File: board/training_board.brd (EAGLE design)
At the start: 68.6 x 53.4 mm, 24 parts, among them J1 MAIN_PWR, Q1 ARDUINOR3-NOIOREF-NOTEXT, Q2 DMN2056U, SW2 PTS645, U1 DRV8871HSOP-8

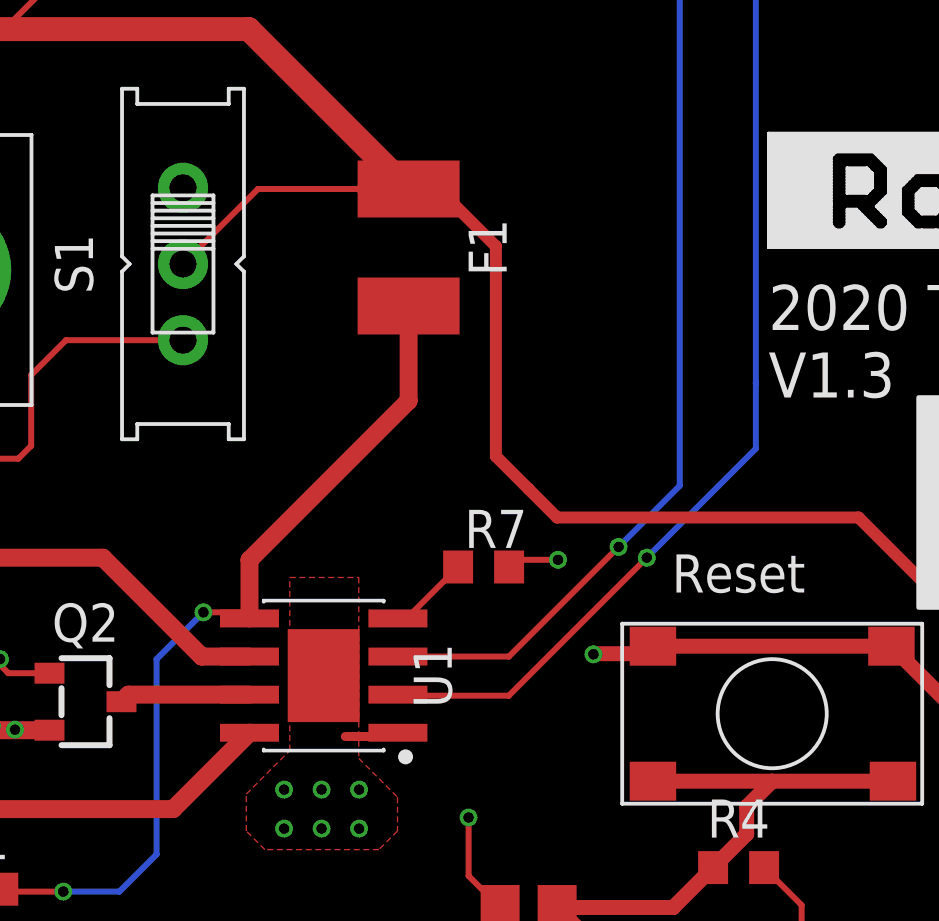
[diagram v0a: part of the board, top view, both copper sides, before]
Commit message: Library updates, slight routing changes
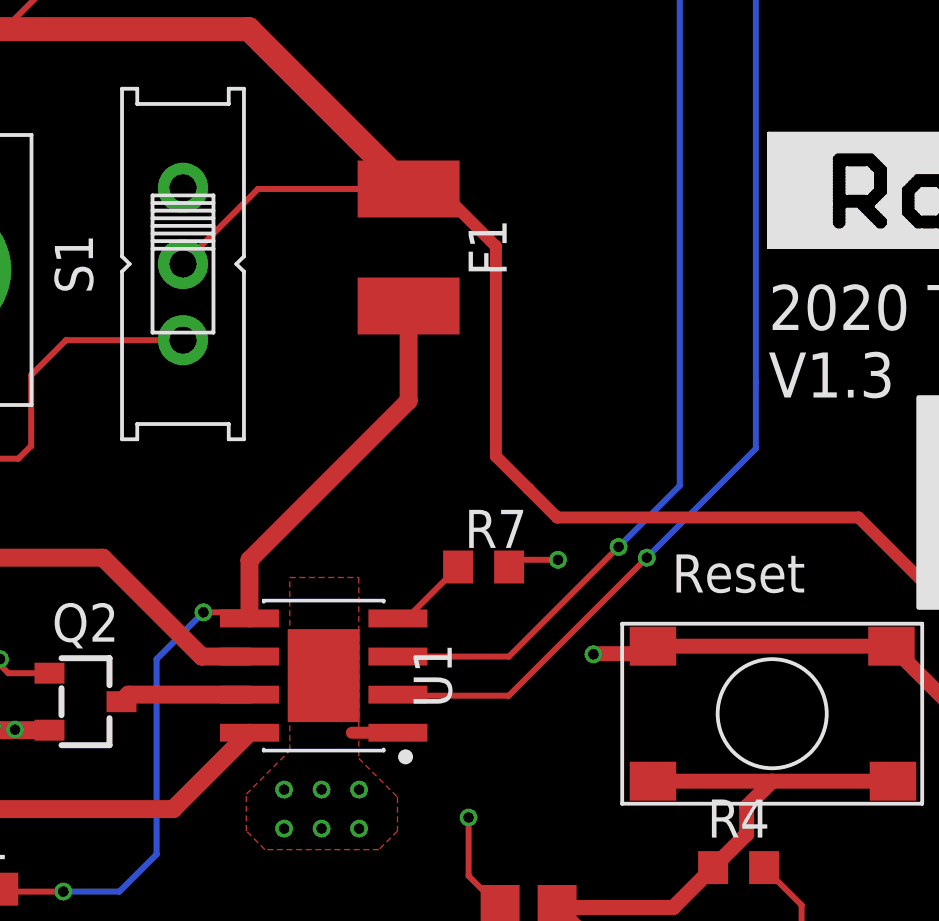
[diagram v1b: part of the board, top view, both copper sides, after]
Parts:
- U1: device RoboJackets-ICs:SOIC127P600X170-9T240X310N -> RoboJackets-ICs:HSOP-8
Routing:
- net +12V: track 92.6 -> 91.1 mm
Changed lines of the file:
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@@
 <elements>
 <element name="Q1" library="adafruit" library_urn="urn:adsk.eagle:library:420" package="ARDUINOR3-NOTEXT-NOIOREF" package3d_urn="urn:adsk.eagle:package:6240888/1" value="ARDUINOR3-NOIOREF-NOTEXT" x="0" y="0" smashed="yes"/>
-<element name="U1" library="RoboJackets-ICs" package="SOIC127P600X170-9T240X310N" package3d_urn="urn:adsk.eagle:package:16996349/1" value="DRV8871HSOP-8" x="22.17" y="12.73" smashed="yes" rot="R180">
+<element name="U1" library="RoboJackets-ICs" package="HSOP-8" value="DRV8871HSOP-8" x="22.17" y="12.73" smashed="yes" rot="R180">
 <attribute name="DKPN" value="296-43024-1-ND" x="22.17" y="12.73" size="1.778" layer="27" rot="R180" display="off"/>
 <attribute name="NAME" x="25.17" y="12.73" size="1.27" layer="25" rot="R270" align="bottom-center"/>
@@
 <vertex x="21.04" y="16"/>
 </polygon>
-<wire x1="24.6434" y1="10.825" x2="24.5184" y2="10.7" width="0.3" layer="1"/>
-<wire x1="24.5184" y1="10.7" x2="22.89" y2="10.7" width="0.3" layer="1"/>
 <via x="20.85" y="8.93" extent="1-16" drill="0.35"/>
 <via x="22.1" y="8.93" extent="1-16" drill="0.35"/>
@@
 <via x="22.1" y="7.63" extent="1-16" drill="0.35"/>
 <via x="20.85" y="7.63" extent="1-16" drill="0.35"/>
+<wire x1="24.6434" y1="10.825" x2="23.105" y2="10.825" width="0.4" layer="1"/>
 </signal>
 <signal name="3V">
@@
 <wire x1="27.91" y1="27.04" x2="26" y2="28.95" width="0.4" layer="1"/>
 <wire x1="26" y1="28.95" x2="25" y2="28.95" width="0.4" layer="1"/>
-<wire x1="23.57" y1="28.95" x2="25" y2="28.95" width="0.6" layer="1"/>
 <wire x1="4.62" y1="34.28" x2="10.62" y2="34.28" width="0.8" layer="1"/>
 <wire x1="10.62" y1="34.28" x2="9.43" y2="33.09" width="0.8" layer="1"/>
@@
 <wire x1="10.62" y1="34.28" x2="19.67" y2="34.28" width="0.8" layer="1"/>
 <wire x1="19.67" y1="34.28" x2="25" y2="28.95" width="0.8" layer="1"/>
-<wire x1="25" y1="28.95" x2="19.98" y2="28.95" width="0.2" layer="1"/>
-<wire x1="19.98" y1="28.95" x2="17.48" y2="26.45" width="0.2" layer="1"/>
+<wire x1="17.48" y1="26.45" x2="19.98" y2="28.95" width="0.2" layer="1"/>
 <wire x1="13.63" y1="36.38" x2="11.53" y2="34.28" width="0.2" layer="1"/>
 <wire x1="11.53" y1="34.28" x2="10.62" y2="34.28" width="0.2" layer="1"/>
 <wire x1="12.08" y1="41.85" x2="13.63" y2="40.3" width="0.2" layer="1"/>
 <wire x1="13.63" y1="40.3" x2="13.63" y2="36.38" width="0.2" layer="1"/>
+<wire x1="19.98" y1="28.95" x2="25" y2="28.95" width="0.2" layer="1"/>
 </signal>
 <signal name="+5V">
@@
 <signal name="M1_FWD">
 <contactref element="Q1" pad="D10"/>
-<wire x1="36.576" y1="22.466" x2="36.576" y2="22.49" width="0.2" layer="16"/>
 <contactref element="U1" pad="2"/>
 <wire x1="36.576" y1="22.49" x2="36.576" y2="50.8" width="0.2" layer="16"/>
@@
 <mfgpreviewcolor name="substratecolor" color="0xFF786E46"/>
 </mfgpreviewcolors>
+<errors>
+</errors>
 </board>
 </drawing>
